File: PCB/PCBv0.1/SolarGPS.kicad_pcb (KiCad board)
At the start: 2 copper layers, 56.3 x 63 mm, 72 parts, among them J1 Conn_01x10_Female, J2 USB_B_Micro, J4 Conn_02x05_Odd_Even, SW1 SW_Push, SW2 SW_Push, U1 BQ25570, U2 MAX-M8Q, U3 STM32L433CCUx, U4 MIC5225, U5 MAX40200AUK, Y1 32.768Hz

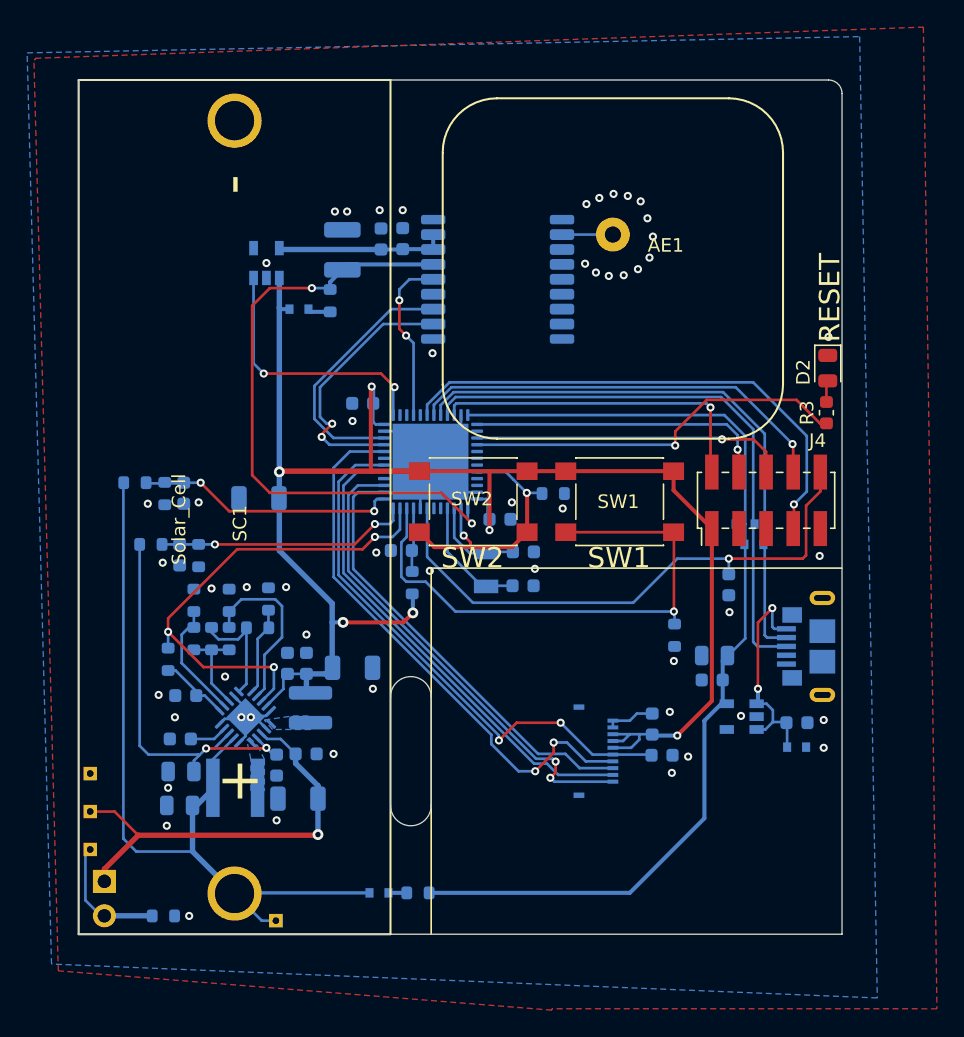
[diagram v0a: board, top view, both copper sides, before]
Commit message: Some dumb changes
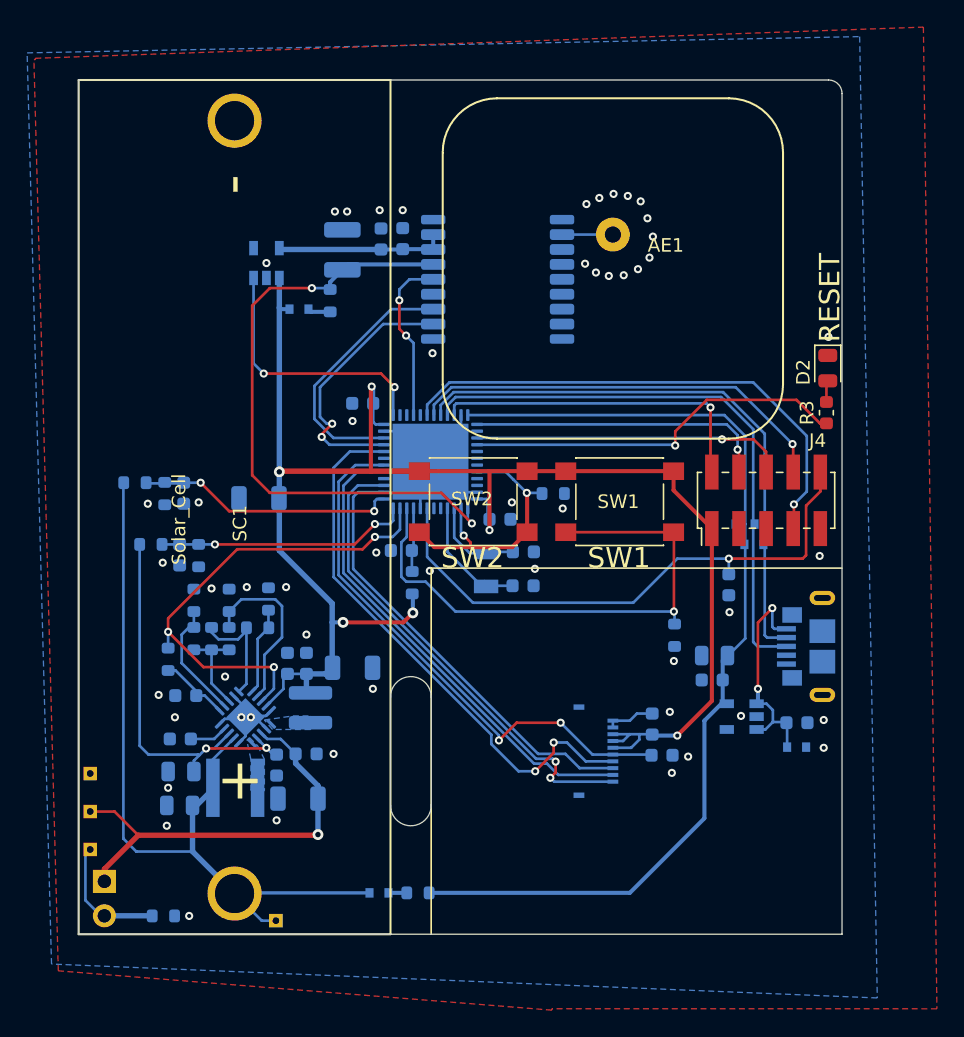
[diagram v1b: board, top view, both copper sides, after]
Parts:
- ROK1: value 5.23M -> 6.49M
- ROK2: value 6.34M -> 5.36M
- ROK3: value 1.27M -> 1M
- ROUT1: value 4.42M -> 5.49M
- ROUT2: value 8.45M -> 7.32M
- ROV1: value 4.32M -> 6.19M
- ROV2: value 8.66M -> 6.65M
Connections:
- J2 pad 4: Net-(J2-Pad4) -> unconnected-(J2-Pad4)
- U2 pad 13: Net-(U2-Pad13) -> unconnected-(U2-Pad13)
- U2 pad 14: Net-(U2-Pad14) -> unconnected-(U2-Pad14)
- U2 pad 15: Net-(U2-Pad15) -> unconnected-(U2-Pad15)
- U2 pad 16: Net-(U2-Pad16) -> unconnected-(U2-Pad16)
- U2 pad 17: Net-(U2-Pad17) -> unconnected-(U2-Pad17)
- U2 pad 18: Net-(U2-Pad18) -> unconnected-(U2-Pad18)
- U2 pad 4: Net-(U2-Pad4) -> unconnected-(U2-Pad4)
- U2 pad 9: Net-(U2-Pad9) -> unconnected-(U2-Pad9)
- U3 pad 16: Net-(U3-Pad16) -> unconnected-(U3-Pad16)
- U3 pad 19: Net-(U3-Pad19) -> unconnected-(U3-Pad19)
- U3 pad 26: Net-(U3-Pad26) -> unconnected-(U3-Pad26)
- U3 pad 27: Net-(U3-Pad27) -> unconnected-(U3-Pad27)
- U3 pad 29: Net-(U3-Pad29) -> unconnected-(U3-Pad29)
- U3 pad 38: Net-(U3-Pad38) -> unconnected-(U3-Pad38)
- U3 pad 41: Net-(U3-Pad41) -> unconnected-(U3-Pad41)
- U3 pad 42: Net-(U3-Pad42) -> unconnected-(U3-Pad42)
- U3 pad 43: Net-(U3-Pad43) -> unconnected-(U3-Pad43)
- U3 pad 45: Net-(U3-Pad45) -> unconnected-(U3-Pad45)
- U3 pad 46: Net-(U3-Pad46) -> unconnected-(U3-Pad46)
- U3 pad 5: Net-(U3-Pad5) -> unconnected-(U3-Pad5)
- U3 pad 6: Net-(U3-Pad6) -> unconnected-(U3-Pad6)
- U4 pad 4: Net-(U4-Pad4) -> unconnected-(U4-Pad4)
- U5 pad 4: Net-(U5-Pad4) -> unconnected-(U5-Pad4)
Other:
- net class Default removed
- net class VDD removed
- net class VREF removed
